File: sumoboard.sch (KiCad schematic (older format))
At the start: 29 parts, among them J1 LEFT_SERVO, J2 RIGHT_SERVO, J3 ULTRASONIC, J4 CONN_02X04, J5 WEMOS, J6 CONN_02X04, P1 WEOMOS_LOLIN32, SW1 ON / OFF

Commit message: sumoboard v0.2
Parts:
- removed BT1: BATTERY, w_conn_jst-ph:b2b-ph-kl, symbol Battery_Cell
- removed P1: WEOMOS_LOLIN32, RoboKoding:WEMOS_LOLIN32, symbol WEOMOS_LOLIN32
- removed R2, R3: R, Resistors_THT:R_Axial_DIN0207_L6.3mm_D2.5mm_P10.16mm_Horizontal, symbol R
- added J7: B+, Pin_Headers:Pin_Header_Straight_1x01_Pitch2.54mm, symbol CONN_01X01
- added J8: B-, Pin_Headers:Pin_Header_Straight_1x01_Pitch2.54mm, symbol CONN_01X01
- added P1: WEOMOS_LOLIN32_LITE, RoboKoding:WEMOS_LOLIN32_LITE, symbol WEOMOS_LOLIN32_LITE
- C1, C2: value CP -> 10V+,800uF+; footprint Capacitors_THT:CP_Radial_D10.0mm_P2.50mm -> Capacitors_ThroughHole:C_Radial_D10_L25_P5
- J4: value CONN_02X04 -> right_bridge
- J5: footprint w_conn_jst-ph:b2b-ph-kl -> Pin_Headers:Pin_Header_Straight_1x02_Pitch2.54mm
- J6: value CONN_02X04 -> left_bridge
- R1, R4, R5, R6, R7: value R -> 100R
- R10, R11: value R -> 100K
- R8, R9: value R -> 0R1
- SW1: footprint Buttons_Switches_THT:SW_Micro_SPST -> Buttons_Switches_ThroughHole:SW_PUSH_x2
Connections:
- net labels added: D15
- net labels removed: D0
- wire segments 110 -> 101
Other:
- note added: "echo"
- note added: "left_line\n"
- note added: "left_servo\n"
- note added: "line_left\n"
- note added: "line_right\n"
- note added: "right_line\n"
- note added: "right_servo"
- note added: "trigger\n"
- note added: "ultrasonic"
- moved on the sheet: C1, C2, J1, J2, J4, J5, J6, R10, R11, R8, R9, SW1

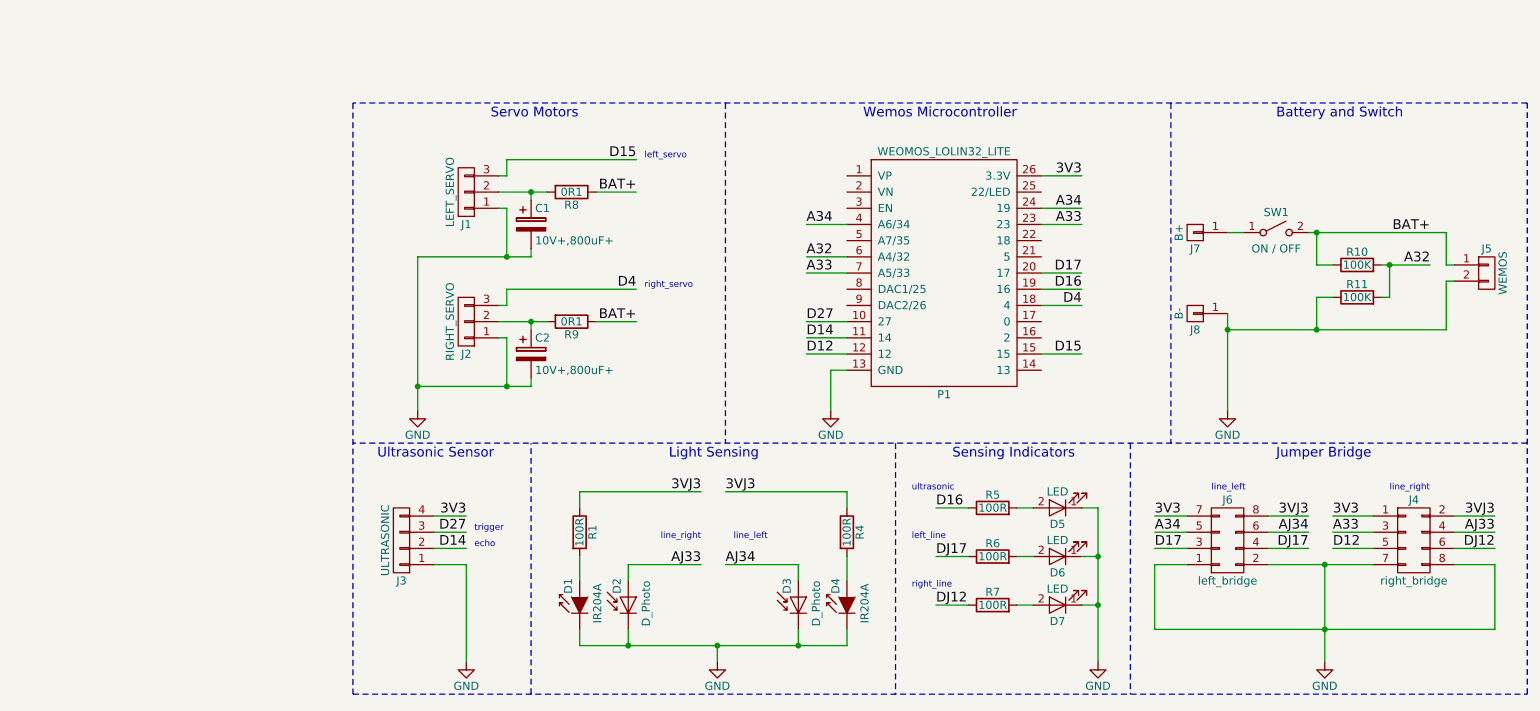
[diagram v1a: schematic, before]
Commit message: update to v0.3.1
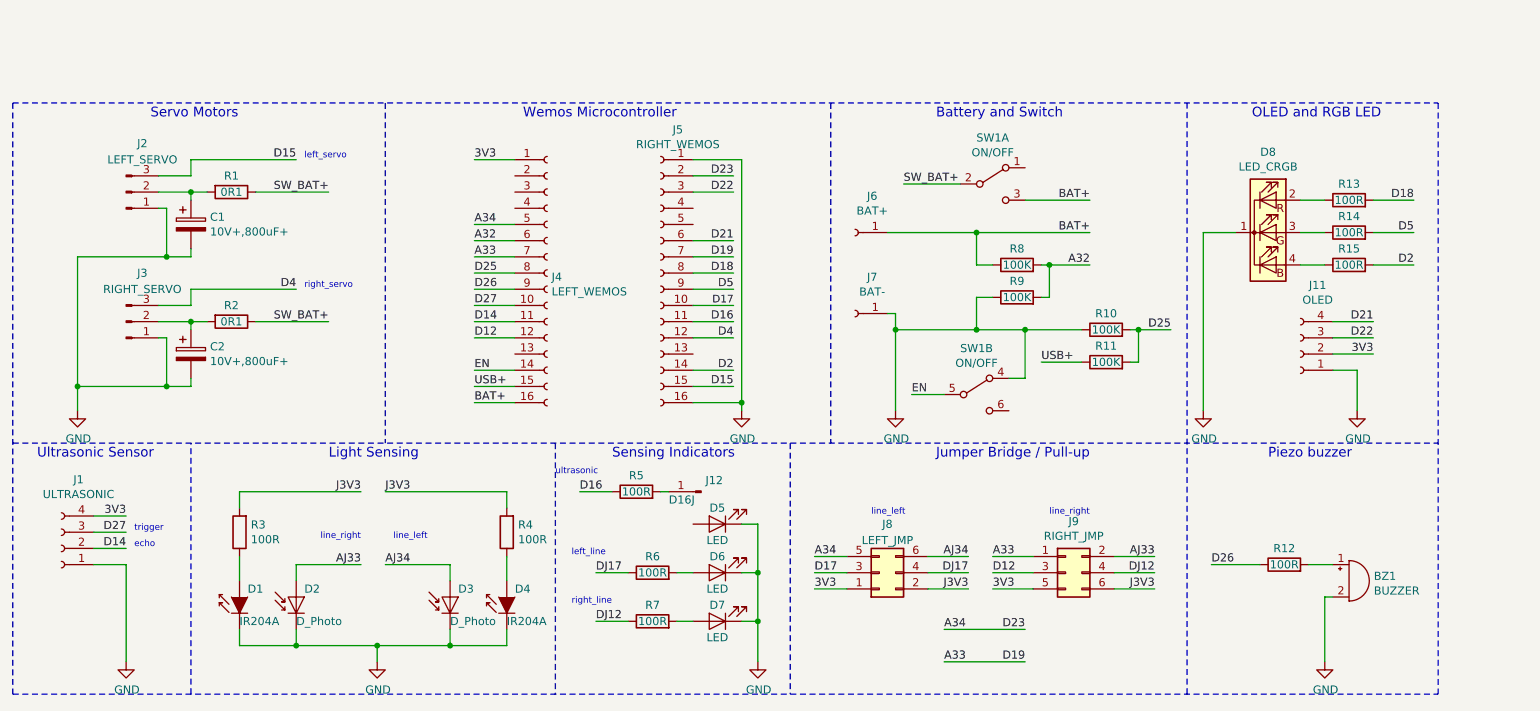
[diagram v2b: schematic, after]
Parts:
- removed C1, C2: 10V+,800uF+, Capacitors_ThroughHole:C_Radial_D10_L25_P5, symbol CP
- removed D1, D4: IR204A, LEDs:LED_D3.0mm, symbol IR204A
- removed D2, D3: D_Photo, LEDs:LED_D3.0mm, symbol D_Photo
- removed D5, D6, D7: LED, LEDs:LED_D5.0mm, symbol LED
- removed J1: LEFT_SERVO, Pin_Headers:Pin_Header_Straight_1x03_Pitch2.54mm, symbol CONN_01X03
- removed J2: RIGHT_SERVO, Pin_Headers:Pin_Header_Straight_1x03_Pitch2.54mm, symbol CONN_01X03
- removed J3: ULTRASONIC, Pin_Headers:Pin_Header_Straight_1x04_Pitch2.54mm, symbol CONN_01X04
- removed J4: right_bridge, Pin_Headers:Pin_Header_Straight_2x04_Pitch2.54mm_SMD, symbol CONN_02X04
- removed J5: WEMOS, Pin_Headers:Pin_Header_Straight_1x02_Pitch2.54mm, symbol CONN_01X02
- removed J6: left_bridge, Pin_Headers:Pin_Header_Straight_2x04_Pitch2.54mm_SMD, symbol CONN_02X04
- removed J7: B+, Pin_Headers:Pin_Header_Straight_1x01_Pitch2.54mm, symbol CONN_01X01
- removed J8: B-, Pin_Headers:Pin_Header_Straight_1x01_Pitch2.54mm, symbol CONN_01X01
- removed P1: WEOMOS_LOLIN32_LITE, RoboKoding:WEMOS_LOLIN32_LITE, symbol WEOMOS_LOLIN32_LITE
- removed R1, R4, R5, R6, R7: 100R, Resistors_THT:R_Axial_DIN0207_L6.3mm_D2.5mm_P10.16mm_Horizontal, symbol R
- removed R10, R11: 100K, Resistors_THT:R_Axial_DIN0207_L6.3mm_D2.5mm_P10.16mm_Horizontal, symbol R
- removed R8, R9: 0R1, Resistors_THT:R_Axial_DIN0207_L6.3mm_D2.5mm_P10.16mm_Horizontal, symbol R
- removed SW1: ON / OFF, Buttons_Switches_ThroughHole:SW_PUSH_x2, symbol SW_SPST
- added BZ1: BUZZER, Buzzer_Beeper:MagneticBuzzer_ProSignal_ABT-410-RC, symbol Device:Buzzer
- added C1, C2: 10V+,800uF+, Capacitor_THT:CP_Radial_D10.0mm_P7.50mm, symbol Device:CP
- added D1, D4: IR204A, LED_THT:LED_D3.0mm_Clear, symbol LED:IR204A
- added D2, D3: D_Photo, LED_THT:LED_D3.0mm_IRBlack, symbol Device:D_Photo
- added D5, D6, D7: LED, LED_THT:LED_D5.0mm, symbol Device:LED
- added D8: LED_CRGB, LED_THT:LED_D5.0mm-4, symbol Device:LED_CRGB
- added J1: ULTRASONIC, Connector_PinSocket_2.54mm:PinSocket_1x04_P2.54mm_Vertical, symbol Connector:Conn_01x04_Female
- added J11: OLED, Connector_PinSocket_2.54mm:PinSocket_1x04_P2.54mm_Vertical, symbol Connector:Conn_01x04_Female
- added J12: D16J, Connector_PinHeader_2.54mm:PinHeader_1x01_P2.54mm_Vertical, symbol Connector:Conn_01x01_Male
- added J2: LEFT_SERVO, Connector_PinHeader_2.54mm:PinHeader_1x03_P2.54mm_Vertical, symbol Connector:Conn_01x03_Male
- added J3: RIGHT_SERVO, Connector_PinHeader_2.54mm:PinHeader_1x03_P2.54mm_Vertical, symbol Connector:Conn_01x03_Male
- added J4: LEFT_WEMOS, Connector_PinSocket_2.54mm:PinSocket_1x16_P2.54mm_Vertical, symbol Connector:Conn_01x16_Female
- added J5: RIGHT_WEMOS, Connector_PinSocket_2.54mm:PinSocket_1x16_P2.54mm_Vertical, symbol Connector:Conn_01x16_Female
- added J6: BAT+, Connector_PinHeader_2.54mm:PinHeader_1x01_P2.54mm_Vertical, symbol Connector:Conn_01x01_Female
- added J7: BAT-, Connector_PinHeader_2.54mm:PinHeader_1x01_P2.54mm_Vertical, symbol Connector:Conn_01x01_Female
- added J8: LEFT_JMP, Connector_PinHeader_2.54mm:PinHeader_2x03_P2.54mm_Vertical, symbol Connector_Generic:Conn_02x03_Odd_Even
- added J9: RIGHT_JMP, Connector_PinHeader_2.54mm:PinHeader_2x03_P2.54mm_Vertical, symbol Connector_Generic:Conn_02x03_Odd_Even
- added R1, R2: 0R1, Resistor_THT:R_Axial_DIN0309_L9.0mm_D3.2mm_P15.24mm_Horizontal, symbol Device:R
- added R10, R11, R8, R9: 100K, Resistor_THT:R_Axial_DIN0207_L6.3mm_D2.5mm_P10.16mm_Horizontal, symbol Device:R
- added R12, R13, R14, R15, R3, R4, R5, R6, R7: 100R, Resistor_THT:R_Axial_DIN0207_L6.3mm_D2.5mm_P10.16mm_Horizontal, symbol Device:R
- added SW1: ON/OFF, Button_Switch_THT:SW_E-Switch_EG2219_DPDT_Angled, symbol Switch:SW_DPDT_x2
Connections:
- net 3V3: now also J1.4 (Pin_4), J11.2 (Pin_2), J4.1 (Pin_1), J8.1 (Pin_1), J9.5 (Pin_5)
- net A32: now also J4.6 (Pin_6), R8.2, R9.2
- net A33: now also J4.7 (Pin_7), J5.7 (Pin_7), J9.1 (Pin_1)
- net A34: now also J4.5 (Pin_5), J5.2 (Pin_2), J8.5 (Pin_5)
- net AJ33: now also D2.2 (A), J9.2 (Pin_2)
- net AJ34: now also D3.2 (A), J8.6 (Pin_6)
- net BAT+: now also J4.16 (Pin_16), J6.1 (Pin_1), R8.1, SW1.3 (C)
- net D12: now also J4.12 (Pin_12), J9.3 (Pin_3)
- net D14: now also J1.2 (Pin_2), J4.11 (Pin_11)
- net D15: now also J2.3 (Pin_3), J5.15 (Pin_15)
- net D16: now also J5.11 (Pin_11), R5.1
- net D17: now also J5.10 (Pin_10), J8.3 (Pin_3)
- net D27: now also J1.3 (Pin_3), J4.10 (Pin_10)
- net D4: now also J3.3 (Pin_3), J5.12 (Pin_12)
- net DJ12: now also J9.4 (Pin_4), R7.1
- net DJ17: now also J8.4 (Pin_4), R6.1
- net GND: now also BZ1.2 (+), C1.2, C2.2, D1.1 (K), D2.1 (K), D3.1 (K), D4.1 (K), D5.1 (K), D6.1 (K), D7.1 (K), D8.1 (K), J1.1 (Pin_1), J11.1 (Pin_1), J2.1 (Pin_1), J3.1 (Pin_1), J5.1 (Pin_1), J5.16 (Pin_16), J7.1 (Pin_1), R10.1, R9.1, SW1.4 (A)
- new net: C1.1, J2.2 (Pin_2), R1.2
- new net: C2.1, J3.2 (Pin_2), R2.2
- new net: D1.2 (A), R3.1
- new net: D4.2 (A), R4.1
- new net: J12.1 (Pin_1), R5.2
- new net: D6.2 (A), R6.2
- new net: D7.2 (A), R7.2
- new net: BZ1.1 (-), R12.2
- new net: D8.2 (RA), R13.1
- new net: D8.3 (GA), R14.1
- new net: D8.4 (BA), R15.1
- new net D18: J5.8 (Pin_8), R13.2
- new net D2: J5.14 (Pin_14), R15.2
- new net D21: J11.4 (Pin_4), J5.6 (Pin_6)
- new net D22: J11.3 (Pin_3), J5.3 (Pin_3)
- new net D25: J4.8 (Pin_8), R10.2, R11.2
- new net D26: J4.9 (Pin_9), R12.1
- new net D5: J5.9 (Pin_9), R14.2
- new net EN: J4.14 (Pin_14), SW1.5 (B)
- new net J3V3: J8.2 (Pin_2), J9.6 (Pin_6), R3.2, R4.2
- new net SW_BAT+: R1.1, R2.1, SW1.2 (B)
- new net USB+: J4.15 (Pin_15), R11.1
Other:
- note added: "Jumper Bridge / Pull-up"
- note added: "OLED and RGB LED"
- note added: "Piezo buzzer"
- note removed: "Jumper Bridge"
